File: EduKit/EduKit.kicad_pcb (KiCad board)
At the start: 2 copper layers, 25 parts, among them P1 Wheel, P10 BlueLED, P11 IRReceiver, P2 Wheel, P3 Sonar, P4 PowerPINs, P5 Headlight, P6 Headlight, P7 RCReader, P8 IRTransmitter, P9 RedLED, U1 L293D, U2 Arduino_Mini, U3 SPX2920U-3.3, U4 ESP8266, U5 PowerButton

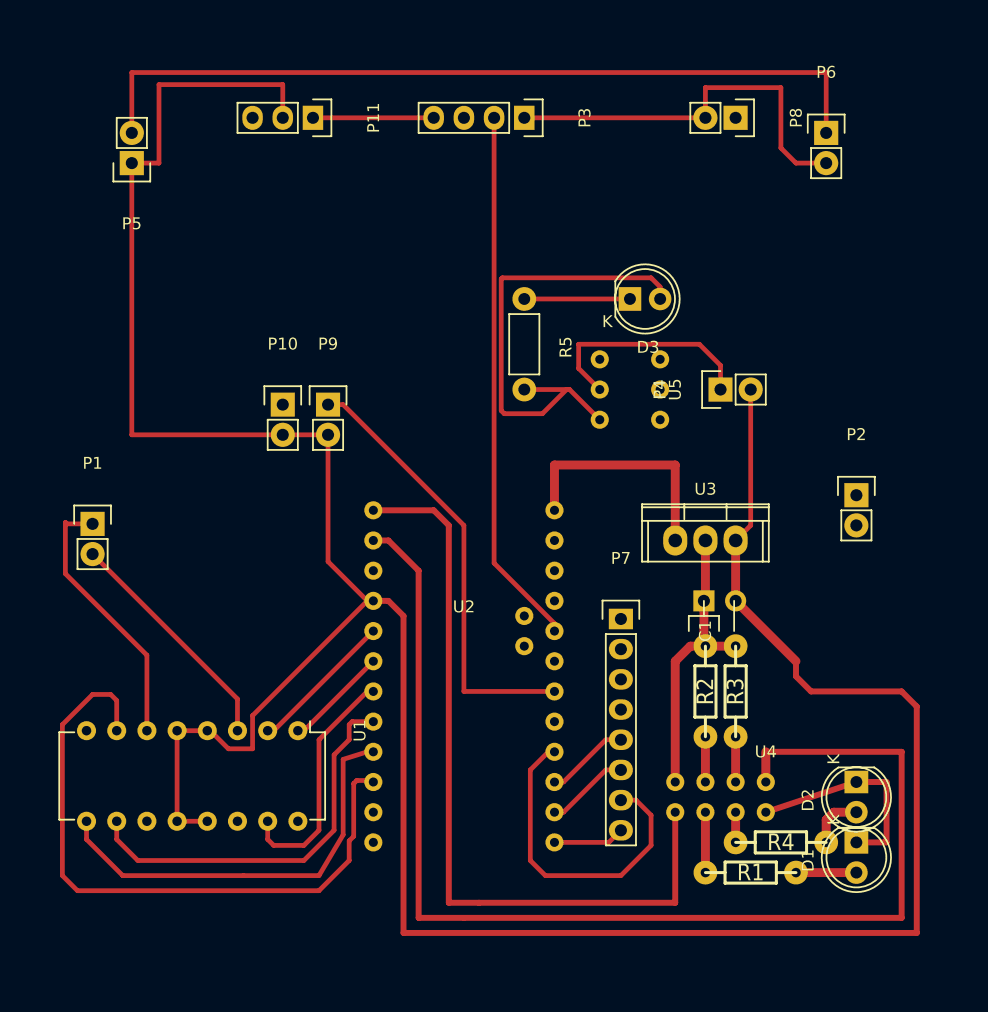
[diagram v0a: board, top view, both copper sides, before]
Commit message: Jackalized a little
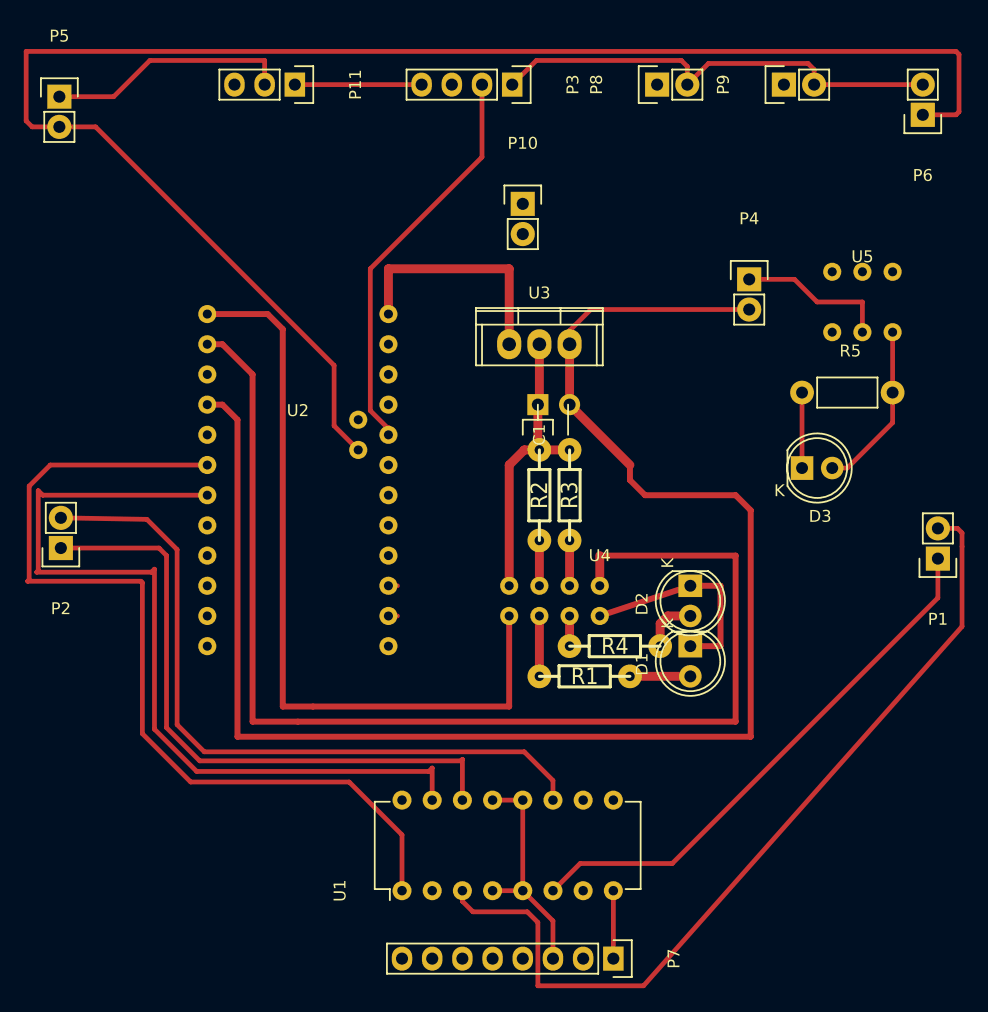
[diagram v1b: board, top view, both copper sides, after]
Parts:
- P10: value BlueLED -> Speaker
- moved P1 71.2 mm to (179.1, 97.8), turned to 180 degrees
- moved P2 67.1 mm to (105.3, 96.9), turned to 180 degrees
- moved P9 46.9 mm to (166.1, 57.9), turned to 90 degrees
- moved P7 28.6 mm to (151.8, 131.4), turned to 270 degrees
- moved P10 26.3 mm to (144.1, 67.9)
- moved R5 24.7 mm to (167.6, 83.8), turned to 0 degrees
- moved U2 21.6 mm to (125.2, 84.8)
- moved C1 21.6 mm to (148.1, 84.8)
- moved D2 21.6 mm to (158.2, 100.1)
- moved R1 21.6 mm to (150.6, 107.7)
- moved U3 21.6 mm to (145.5, 79.8)
- moved U4 21.6 mm to (148.1, 102.6)
- moved D1 21.6 mm to (158.2, 105.2)
- moved R2 21.6 mm to (145.5, 92.5)
- moved R3 21.6 mm to (148.1, 92.5)
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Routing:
- net Net-(U1-Pad1): track 8.77 -> 76.2 mm
- net Net-(P5-Pad2): track 68.6 -> 134.8 mm
- net Net-(P10-Pad2): track 146.2 -> 81.7 mm
- net Net-(P2-Pad2): track 0.00 -> 60.8 mm
- net Net-(U1-Pad7): track 55.2 -> 0.18 mm
- net Net-(P2-Pad1): track 0.00 -> 53.2 mm
- net Net-(P1-Pad2): track 19.9 -> 72.7 mm
- net Net-(U1-Pad15): track 21.0 -> 73.4 mm
- net Net-(P9-Pad1): track 37.2 -> 0.00 mm
- net Net-(U1-Pad9): track 35.3 -> 0.51 mm
- net Net-(U1-Pad10): track 33.2 -> 0.00 mm
- net Net-(P7-Pad7): track 27.6 -> 0.51 mm
- net Net-(D3-Pad2): track 60.0 -> 34.6 mm
- net Net-(P1-Pad1): track 22.7 -> 45.9 mm
- net Net-(U1-Pad2): track 12.4 -> 0.00 mm
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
